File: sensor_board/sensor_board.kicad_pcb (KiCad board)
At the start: 2 copper layers, 10.2 x 10.2 mm, 4 parts, among them U1 TSL25911FN

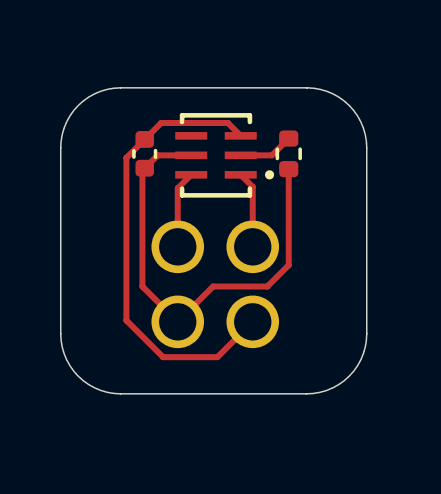
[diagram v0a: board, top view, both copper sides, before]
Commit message: layout edits
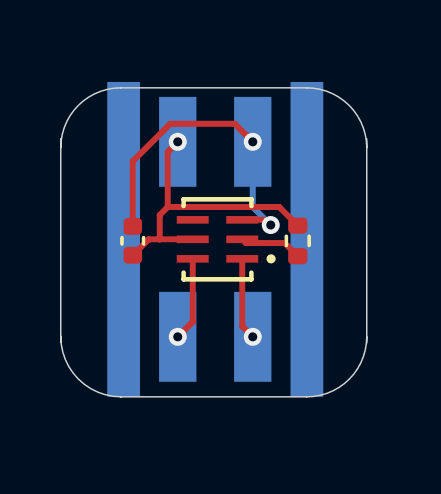
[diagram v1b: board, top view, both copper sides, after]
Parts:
- BlackbodyC1: footprint blackbodies:CONN_SD-105310-100_04_MOL -> blackbodies:CONN_SD-105429-001_04_MOL
- moved C4 2.93 mm to (107.2, 53.7)
- moved R1 2.92 mm to (112.7, 53.7), turned to -90 degrees
- moved U1 2.80 mm to (110.0, 53.7)
- moved BlackbodyC1 1.27 mm to (110.0, 53.7)
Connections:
- BlackbodyC1 pad 1: /SDA -> /SCL
- BlackbodyC1 pad 2: /SCL -> /SDA
- BlackbodyC1 pad 3: +3V3 -> GND
- BlackbodyC1 pad 4: GND -> +3V3
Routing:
- net +3V3: track 15.0 -> 10.3 mm, vias 0 -> 1
- net GND: track 15.1 -> 11.1 mm, vias 0 -> 2
- net /SDA: track 2.59 -> 2.81 mm, vias 0 -> 1
- net /SCL: track 2.57 -> 2.74 mm, vias 0 -> 1
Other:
- board size 10.2 x 10.2 mm -> 10.2 x 10.3 mm

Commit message: layout updates
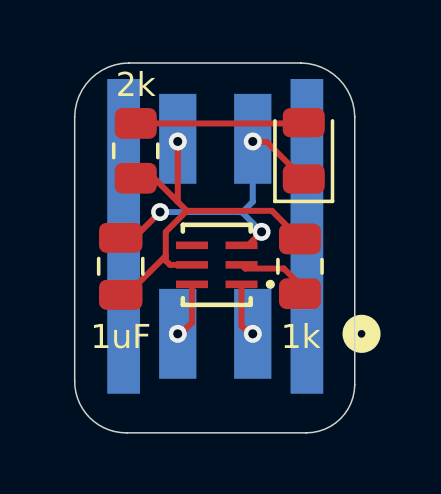
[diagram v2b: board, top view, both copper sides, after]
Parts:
- added Power1: D, LED_SMD:LED_0805_2012Metric, F.Cu at (112.9, 50.7)
- added R2: 2k, Resistor_SMD:R_0805_2012Metric, F.Cu at (107.3, 50.7)
- C4: footprint Capacitor_SMD:C_0402_1005Metric -> Capacitor_SMD:C_0805_2012Metric
- R1: footprint Resistor_SMD:R_0402_1005Metric -> Resistor_SMD:R_0805_2012Metric
- moved C4 0.94 mm to (106.8, 54.5)
- moved R1 0.85 mm to (112.8, 54.5)
- moved U1 0.85 mm to (110.0, 54.5)
- moved BlackbodyC1 0.10 mm to (110.0, 53.5)
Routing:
- net Net-(Power1-A): track 0.00 -> 5.61 mm
- net +3V3: track 10.3 -> 13.2 mm
- net /SDA: track 2.81 -> 1.91 mm
- net /SCL: track 2.74 -> 1.86 mm
- net GND: vias 2 -> 3
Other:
- board size 10.2 x 10.3 mm -> 9.3 x 12.3 mm
